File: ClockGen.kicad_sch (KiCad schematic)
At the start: 21 parts, among them Q1 2N4258, Q2 2N4258, Y1 XT0001

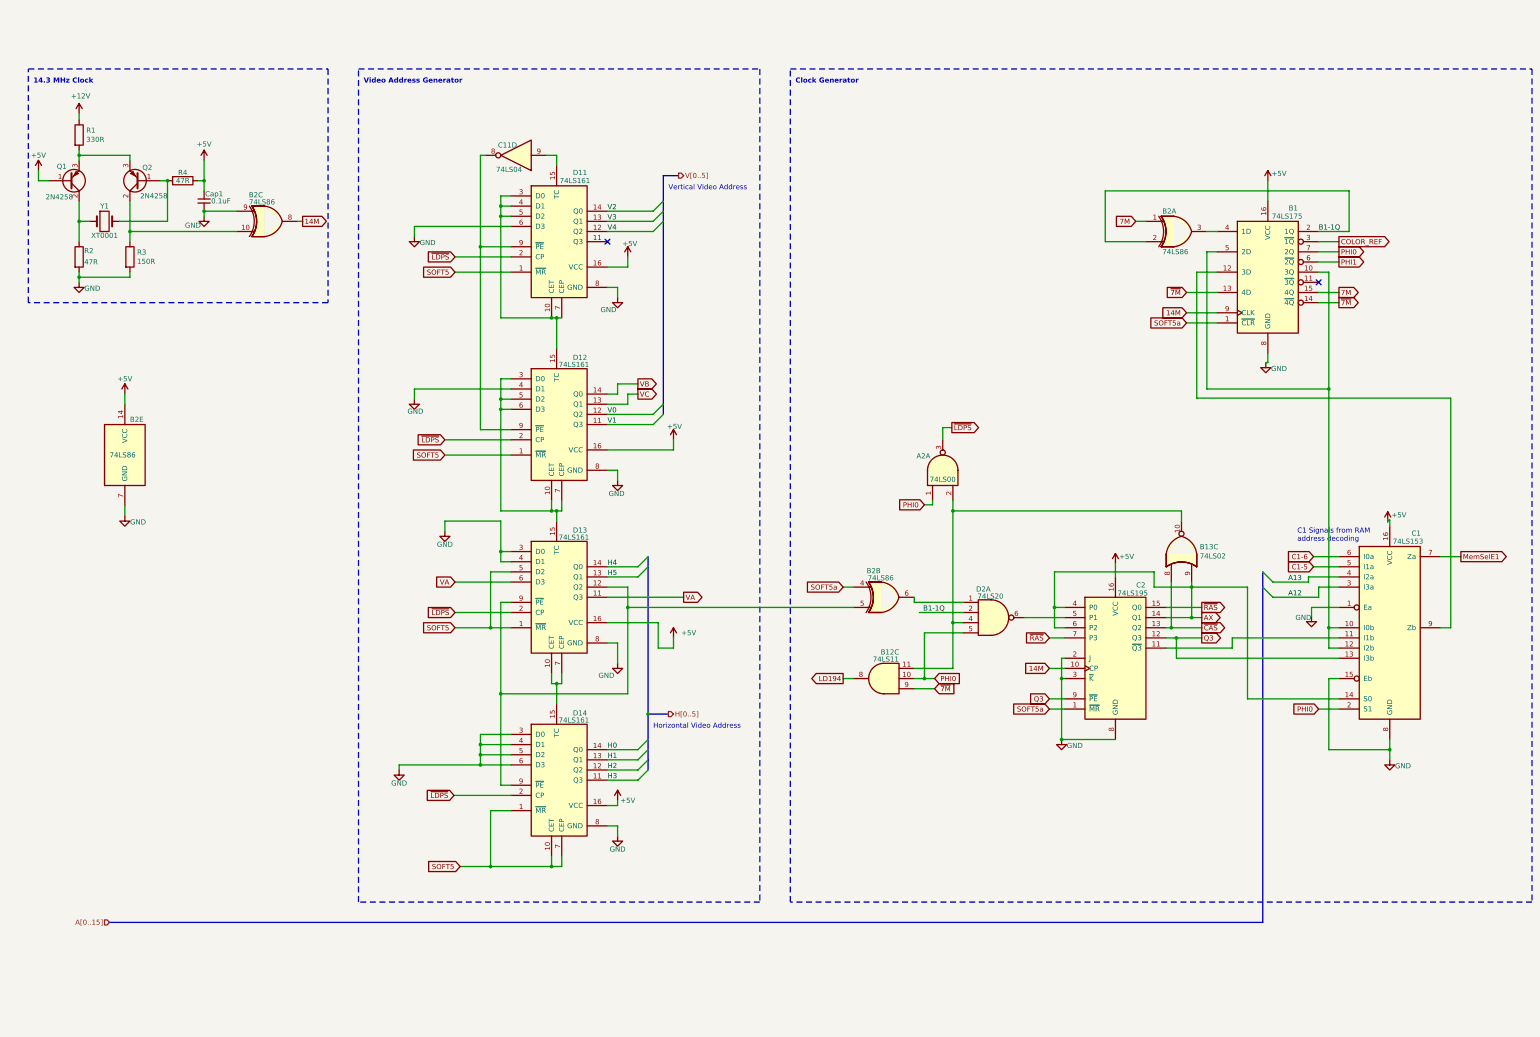
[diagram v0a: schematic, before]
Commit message: Add files via upload
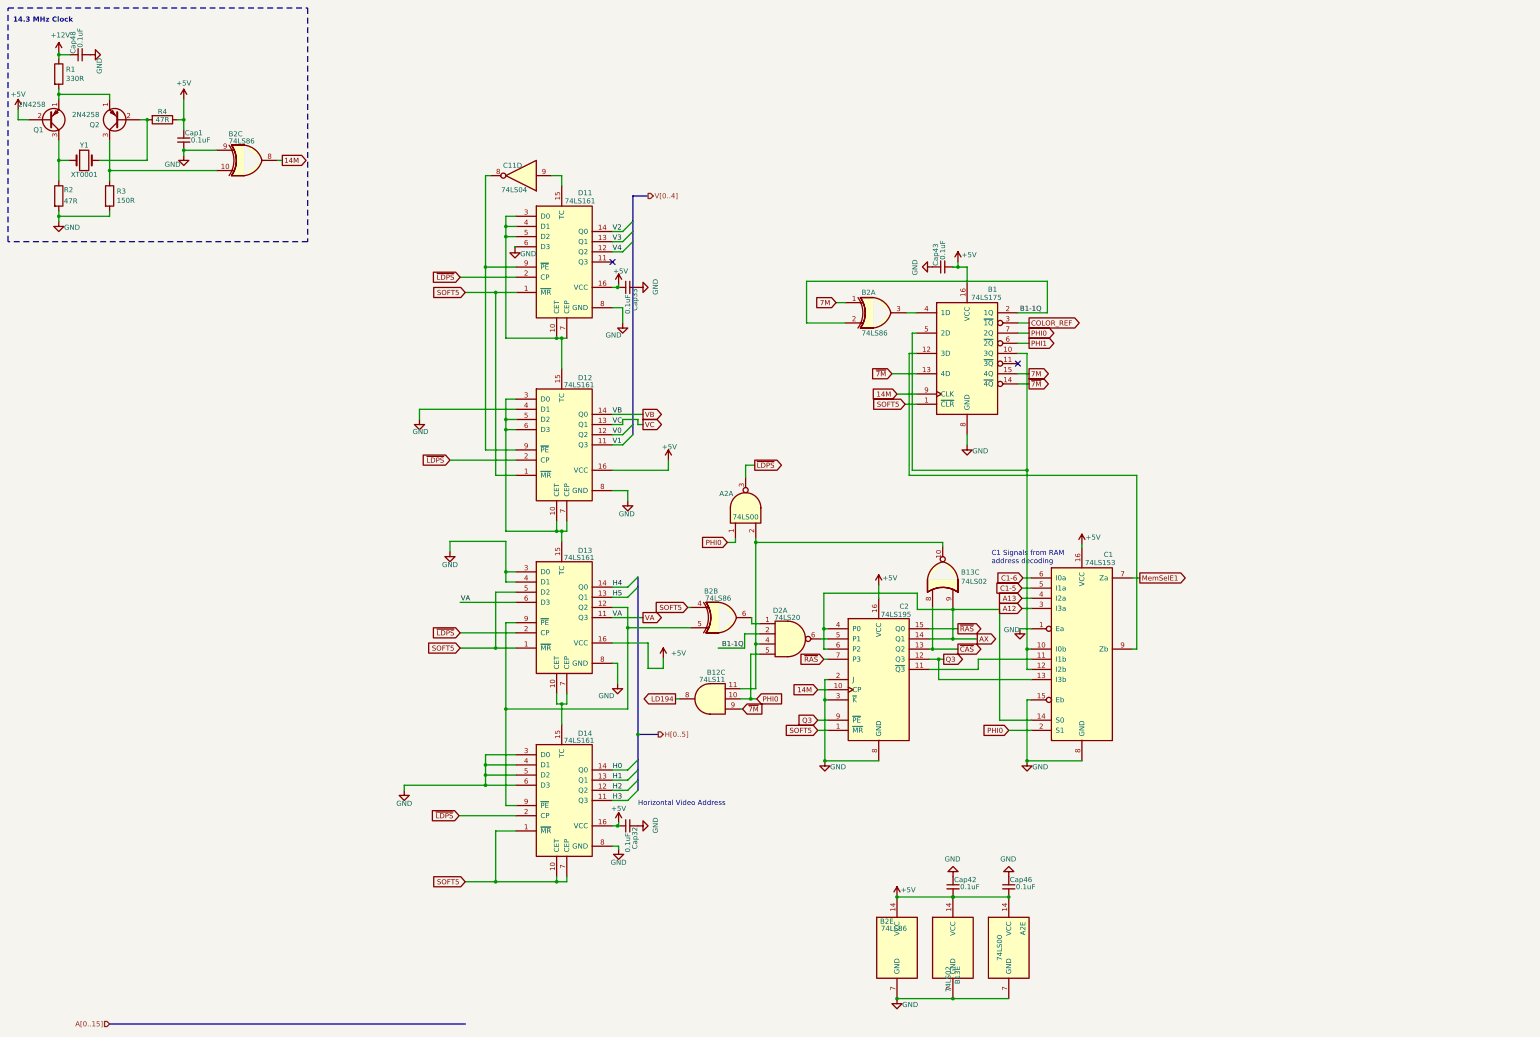
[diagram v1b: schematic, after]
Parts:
- removed Q1, Q2: 2N4258, symbol Device:Q_PNP_BCE
- added unit 5 of A2
- added unit 5 of B13
- added Cap32, Cap33, Cap42, Cap43, Cap46, Cap48: 0.1uF, Apple-II:C_Disc_D5.0mm_W2.5mm_P5.00mm, symbol Device:C_Small
- added Q1, Q2: 2N4258, Package_TO_SOT_THT:TO-18-3, symbol Device:Q_PNP_EBC
- A2, B12, B13, B2, C11, D2: footprint Apple:DIP-14_W7.62mm -> Package_DIP:DIP-14_W7.62mm
- B1, C1, C2, D11, D12, D13, D14: footprint Apple:DIP-16_W7.62mm -> Package_DIP:DIP-16_W7.62mm
- B2: footprint (none) -> Package_DIP:DIP-14_W7.62mm
- Cap1: footprint (none) -> Apple-II:C_Disc_D5.0mm_W2.5mm_P5.00mm
- R1, R2, R3, R4: footprint Resistor_THT:R_Axial_DIN0207_L6.3mm_D2.5mm_P10.16mm_Horizontal -> Apple-II:R_Axial_DIN0207_L6.3mm_D2.5mm_P10.16mm_Horizontal
- Y1: footprint (none) -> Crystal:Crystal_HC18-U_Vertical
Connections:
- net SOFT5a is gone; now on net SOFT5: B1.1 (~{CLR}), B2.4, C2.1 (~{MR})
- net +12V: now also Cap48.1
- net +5V: now also A2.14 (VCC), B13.14 (VCC), Cap32.2, Cap33.2, Cap42.2, Cap43.2, Cap46.2, Q1.2 (B)
- net GND: now also A2.7 (GND), B13.7 (GND), Cap32.1, Cap33.1, Cap42.1, Cap43.1, Cap46.1, Cap48.2
- net at R4.2, Y1.2: now also Q2.2 (B)
- net at B2.10, R3.1: now also Q2.3 (C)
- net at R1.2: now also Q1.1 (E), Q2.1 (E)
- net at R2.1, Y1.1: now also Q1.3 (C)
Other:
- note removed: "Clock Generator"
- note removed: "Vertical Video Address"
- note removed: "Video Address Generator"
- moved on the sheet: A2A, B1, B12C, B13C, B2A, B2B, B2C, C1, C11D, C2, Cap1, D11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
